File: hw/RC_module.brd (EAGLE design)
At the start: 25 x 45 mm, 42 parts, among them J1 GROVE-4P-2.0-3470130P1, J2 GROVE-4P-2.0-3470130P1, X1 22-23-2021

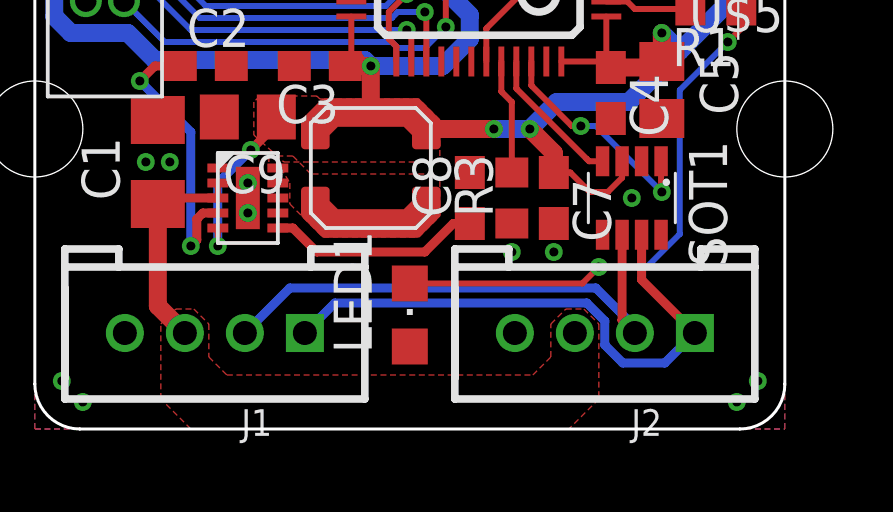
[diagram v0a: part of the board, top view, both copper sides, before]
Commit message: Added logo to bottom silkscreen
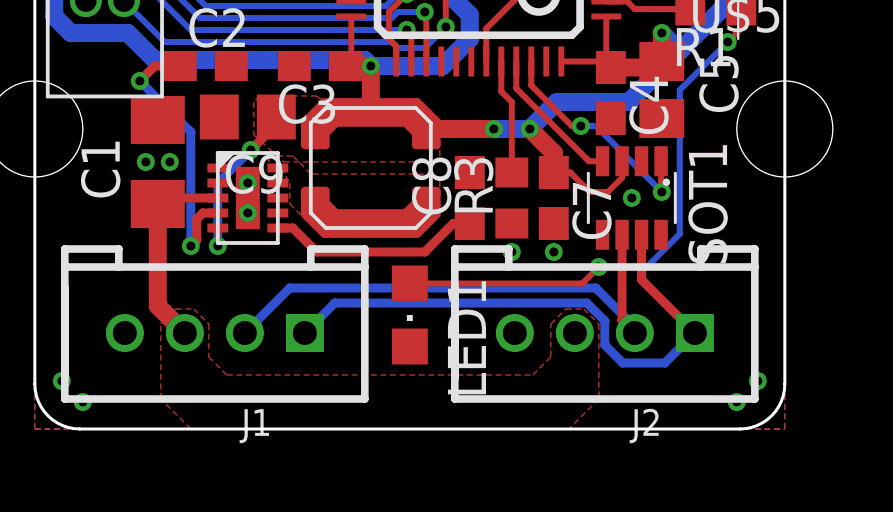
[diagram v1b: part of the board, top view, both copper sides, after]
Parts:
- turned LED1 to 180 degrees
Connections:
- net GND: now also LED1.C; no longer LED1.A
- net N$4: now also LED1.A; no longer LED1.C
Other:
- board text added: "RC module v1.1 (2014/12)"
- board text removed: "RC module rev 1.1"
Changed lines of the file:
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@@
 <grid distance="0.5" unitdist="mm" unit="mm" style="dots" multiple="1" display="yes" altdistance="0.1" altunitdist="mm" altunit="mm"/>
 <layers>
-<layer number="1" name="Top" color="4" fill="1" visible="no" active="yes"/>
-<layer number="16" name="Bottom" color="1" fill="1" visible="yes" active="yes"/>
+<layer number="1" name="Top" color="4" fill="1" visible="yes" active="yes"/>
+<layer number="16" name="Bottom" color="1" fill="1" visible="no" active="yes"/>
 <layer number="17" name="Pads" color="2" fill="1" visible="yes" active="yes"/>
 <layer number="18" name="Vias" color="2" fill="1" visible="yes" active="yes"/>
 <layer number="19" name="Unrouted" color="6" fill="1" visible="yes" active="yes"/>
 <layer number="20" name="Dimension" color="15" fill="1" visible="yes" active="yes"/>
-<layer number="21" name="tPlace" color="7" fill="1" visible="no" active="yes"/>
-<layer number="22" name="bPlace" color="7" fill="1" visible="yes" active="yes"/>
-<layer number="23" name="tOrigins" color="15" fill="1" visible="no" active="yes"/>
-<layer number="24" name="bOrigins" color="15" fill="1" visible="yes" active="yes"/>
+<layer number="21" name="tPlace" color="7" fill="1" visible="yes" active="yes"/>
+<layer number="22" name="bPlace" color="7" fill="1" visible="no" active="yes"/>
+<layer number="23" name="tOrigins" color="15" fill="1" visible="yes" active="yes"/>
+<layer number="24" name="bOrigins" color="15" fill="1" visible="no" active="yes"/>
 <layer number="25" name="tNames" color="7" fill="1" visible="no" active="yes"/>
 <layer number="26" name="bNames" color="7" fill="1" visible="no" active="yes"/>
@@
 <layer number="37" name="tTest" color="7" fill="1" visible="no" active="yes"/>
 <layer number="38" name="bTest" color="7" fill="1" visible="no" active="yes"/>
-<layer number="39" name="tKeepout" color="4" fill="11" visible="no" active="yes"/>
-<layer number="40" name="bKeepout" color="1" fill="11" visible="yes" active="yes"/>
-<layer number="41" name="tRestrict" color="4" fill="10" visible="no" active="yes"/>
-<layer number="42" name="bRestrict" color="1" fill="10" visible="yes" active="yes"/>
+<layer number="39" name="tKeepout" color="4" fill="11" visible="yes" active="yes"/>
+<layer number="40" name="bKeepout" color="1" fill="11" visible="no" active="yes"/>
+<layer number="41" name="tRestrict" color="4" fill="10" visible="yes" active="yes"/>
+<layer number="42" name="bRestrict" color="1" fill="10" visible="no" active="yes"/>
 <layer number="43" name="vRestrict" color="2" fill="10" visible="no" active="yes"/>
 <layer number="44" name="Drills" color="7" fill="1" visible="no" active="yes"/>
@@
 <layer number="46" name="Milling" color="3" fill="1" visible="yes" active="yes"/>
 <layer number="47" name="Measures" color="7" fill="1" visible="yes" active="yes"/>
-<layer number="48" name="Document" color="7" fill="1" visible="no" active="yes"/>
+<layer number="48" name="Document" color="7" fill="1" visible="yes" active="yes"/>
 <layer number="49" name="Reference" color="7" fill="1" visible="no" active="yes"/>
 <layer number="50" name="dxf" color="7" fill="1" visible="no" active="no"/>
-<layer number="51" name="tDocu" color="7" fill="1" visible="no" active="yes"/>
+<layer number="51" name="tDocu" color="7" fill="1" visible="yes" active="yes"/>
 <layer number="52" name="bDocu" color="7" fill="1" visible="no" active="yes"/>
 <layer number="53" name="tGND_GNDA" color="7" fill="1" visible="no" active="no"/>
@@
 <layer number="152" name="_bDocu" color="7" fill="1" visible="no" active="no"/>
 <layer number="199" name="Contour" color="7" fill="1" visible="no" active="yes"/>
-<layer number="200" name="200bmp" color="7" fill="1" visible="yes" active="yes"/>
+<layer number="200" name="200bmp" color="7" fill="1" visible="no" active="yes"/>
 <layer number="201" name="201bmp" color="7" fill="1" visible="no" active="yes"/>
 <layer number="202" name="202bmp" color="7" fill="1" visible="no" active="yes"/>
@@
 <text x="23.6" y="44.3" size="1" layer="20" rot="R180">- S +</text>
 <text x="4" y="6" size="1.5" layer="200" rot="MR90">RC module
-rev 1.1</text>
+v1.1 (2014/12)</text>
 </plain>
 <attributes>
@@
 <element name="C3" library="rcl" package="C0603" value="100n" x="9.5" y="12.1" rot="R180"/>
 <element name="C7" library="rcl" package="C0603" value="100n" x="17.3" y="7.7" rot="R270"/>
-<element name="LED1" library="led" package="CHIPLED_0805" value="" x="12.5" y="3.8"/>
+<element name="LED1" library="led" package="CHIPLED_0805" value="" x="12.5" y="3.8" rot="R180"/>
 <element name="R1" library="rcl" package="R0603" value="330" x="22.7" y="14" rot="R180"/>
 <element name="U$4" library="samtec" package="FTSH-105-TH" value="FTSH-105TH" x="1.7" y="16.8" rot="R270"/>
@@
 <via x="7.1" y="8.2" extent="1-16" drill="0.3"/>
 <via x="7.1" y="7.2" extent="1-16" drill="0.3"/>
-<contactref element="LED1" pad="A"/>
 <contactref element="SOT1" pad="2"/>
 <contactref element="SOT1" pad="8"/>
@@
 <contactref element="JP7" pad="1"/>
 <contactref element="C10" pad="-"/>
+<contactref element="LED1" pad="C"/>
 </signal>
 <signal name="VIN">
@@
 <signal name="N$4">
 <contactref element="R1" pad="1"/>
-<contactref element="LED1" pad="C"/>
 <via x="23.1" y="12.9" extent="1-16" drill="0.3"/>
 <wire x1="23.55" y1="14" x2="23.55" y2="13.35" width="0.2" layer="1"/>
 <wire x1="23.55" y1="13.35" x2="23.1" y2="12.9" width="0.2" layer="1"/>
-<wire x1="12.5" y1="4.85" x2="18.25" y2="4.85" width="0.2" layer="1"/>
 <wire x1="18.25" y1="4.85" x2="18.8" y2="5.4" width="0.2" layer="1"/>
 <via x="18.8" y="5.4" extent="1-16" drill="0.3"/>
@@
 <wire x1="21.5" y1="6.5" x2="21.5" y2="11.3" width="0.2" layer="16"/>
 <wire x1="21.5" y1="11.3" x2="23.1" y2="12.9" width="0.2" layer="16"/>
+<contactref element="LED1" pad="A"/>
+<wire x1="18.25" y1="4.85" x2="12.5" y2="4.85" width="0.2" layer="1"/>
 </signal>
 <signal name="N$2">
